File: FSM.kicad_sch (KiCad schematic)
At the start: 4 parts, among them U20 74HCT74, U22 74HCT00, U23 74HCT00, U9 74HCT04

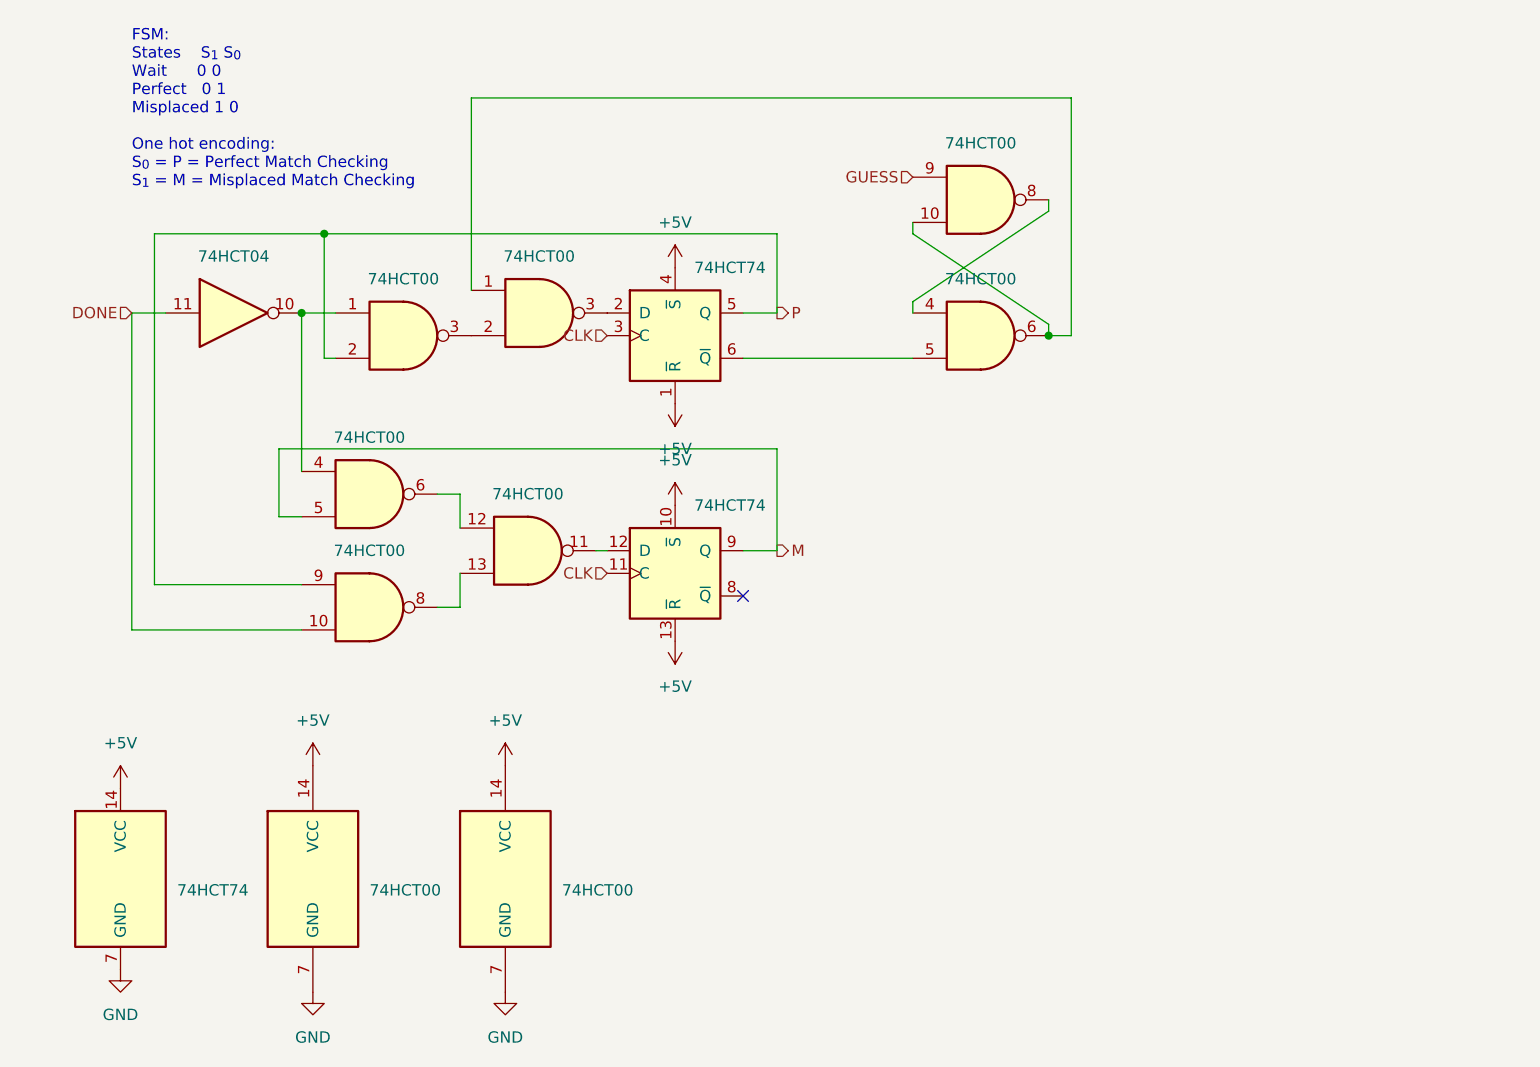
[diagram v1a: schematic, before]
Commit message: Fixes
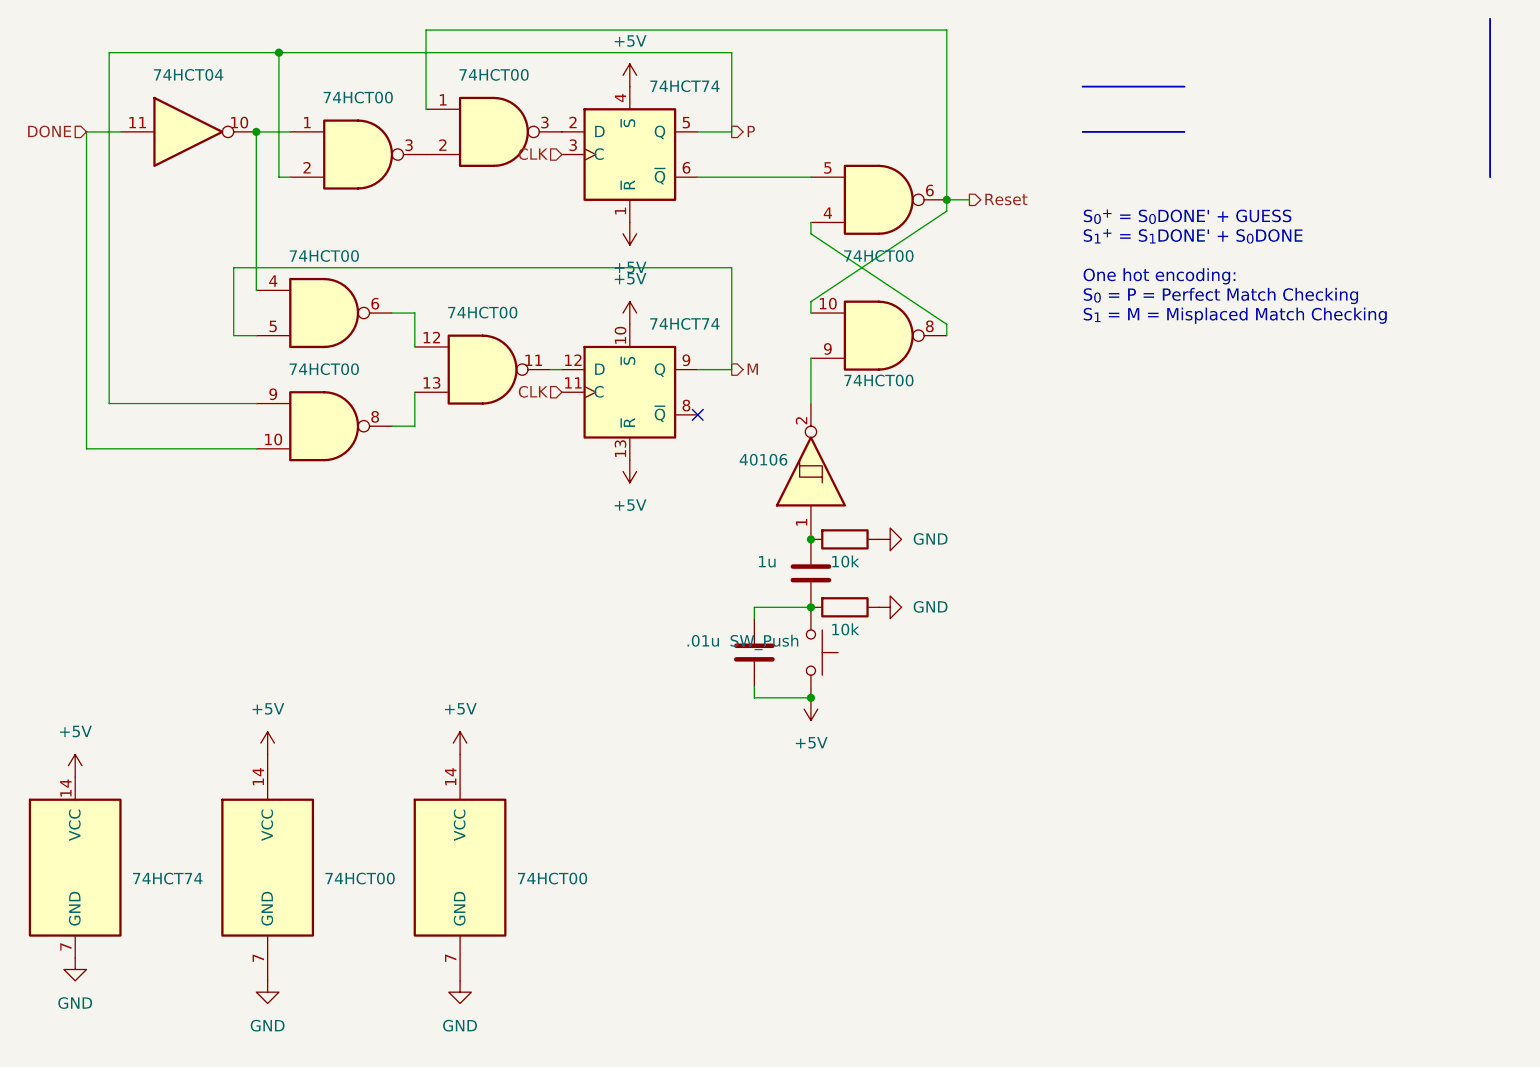
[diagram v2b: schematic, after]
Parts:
- added C3: 1u, symbol Device:C
- added C4: .01u, symbol Device:C
- added R3, R4: 10k, symbol Device:R
- added SW1: SW_Push, symbol Switch:SW_Push
- added U201: 40106, symbol 4xxx:40106
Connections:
- net +5V: now also C4.1, SW1.2
- net GND: now also R3.1, R4.1
- net Reset: now reaches U23.1, U23.10, U23.6
- net GUESS: no longer names the net of U23.9
- net GUESS: now also U201.2
- new net: C3.2, R4.2, U201.1
- new net: C3.1, C4.2, R3.2, SW1.1
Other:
- note added: "S_{0}^{+} = S_{0}DONE' + GUESS S_{1}^{+} = S_{1}DONE' + S_{0}DONE One hot encoding: S_{0} = P = Perfect Match Checking S_{1} = M = Misplaced Match Checking"
- note removed: "FSM: States S_{1} S_{0} Wait 0 0 Perfect 0 1 Misplaced 1 0 One hot encoding: S_{0} = P = Perfect Match Checking S_{1} = M = Misplaced Match Checking"
